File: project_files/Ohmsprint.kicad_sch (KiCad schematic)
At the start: 123 parts, among them J2 MEM2067-02-180-00-A, J3 PJ-002AH-SMT-TR, J4 SJ-3523-SMT-TR, J5 541324062, J6 USB4110-GF-A, Q1 SS8050, Q2 SS8050, Q3 AO3400A, SW1 SW_Push_1_Red, SW2 SW_Push_1_Red, SW3 SW_Push_2_Blue, U1 ESP32-WROOM-32E-N4, U2 AP63203WU, U3 AP63200WU, U4 ATM90E26-YU, U5 ABS210-13, U6 CP2102N-A02-GQFN28R, U7 MCP1727-3302E/SN, U8 TPS2121RUXR, U9 NHD-2.4-240320AF-CSXP, Y1 ABLS-8.192MHZ-B2-T

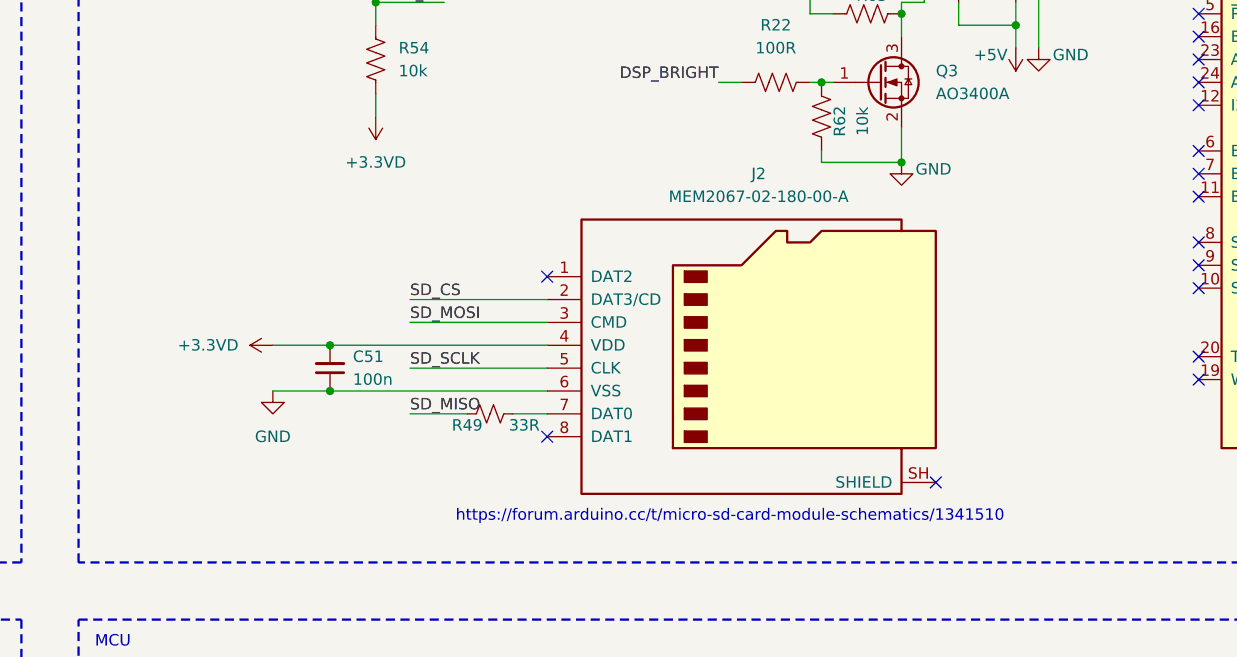
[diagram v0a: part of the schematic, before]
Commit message: Generisani Gerber i Drill
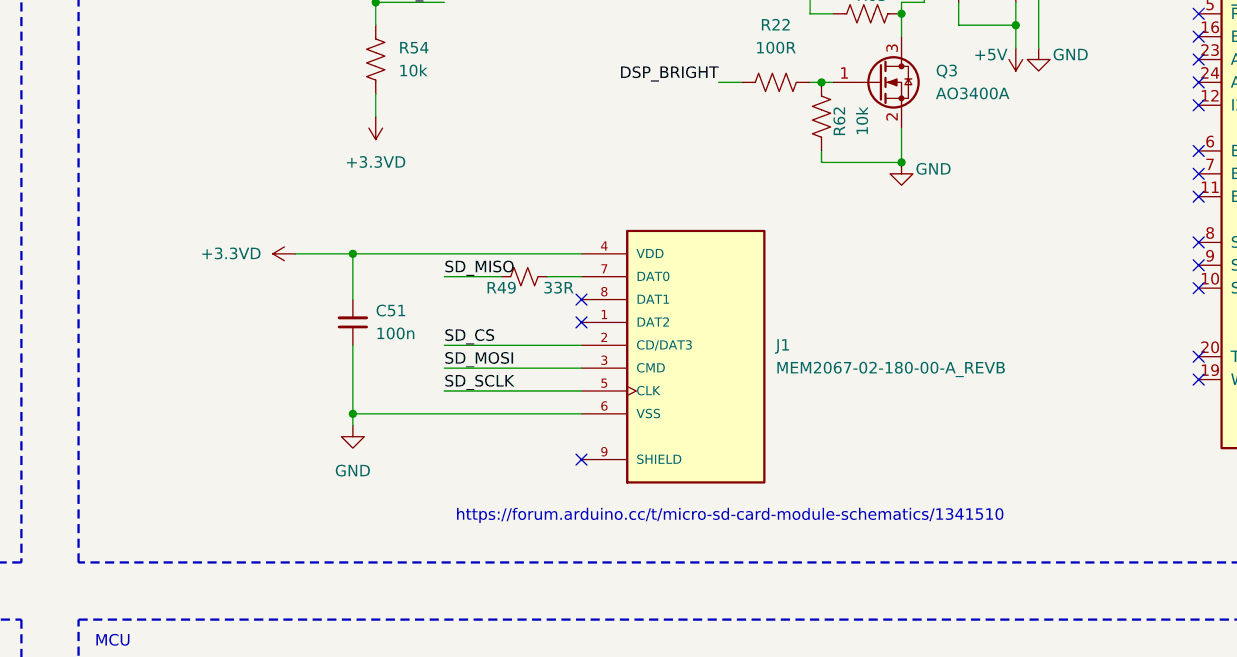
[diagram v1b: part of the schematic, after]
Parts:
- removed J2: MEM2067-02-180-00-A, usb:CONN_MEM2067-02-180-00-A_GCT, symbol Connector:Micro_SD_Card
- added J1: MEM2067-02-180-00-A_REVB, MEM2067-02-180-00-A_REVB_foot:GCT_MEM2067-02-180-00-A_REVB, symbol MEM2067-02-180-00-A_REVB:MEM2067-02-180-00-A_REVB
- J3: footprint PJ_002AH:PJ-002AH-SMT-TR_CUD -> CUI_PJ-002AH-SMT-TR-foot:CUI_PJ-002AH-SMT-TR
- J4: footprint SJ_3523_SMT:SJ-3523-SMT_CUD -> CUI_SJ-3523-SMT-TR-foot:CUI_SJ-3523-SMT-TR
- J5: footprint 541324062:CON_541324062_MOL -> Molex0541324062-foot:CON_541324062_MOL
- U1: footprint esp32_custom:ESP32-WROOM-32D -> RF_Module:ESP32-WROOM-32D
- U8: footprint TPS2121RUXR:RUX0012A -> TPS2121RUXR-foot:RUX0012A
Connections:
- net +3.3VD: now also J1.4 (VDD)
- net GND: now also J1.6 (VSS)
- net SD_CS: now also J1.2 (CD/DAT3)
- net SD_MOSI: now also J1.3 (CMD)
- net SD_SCLK: now also J1.5 (CLK)
- net at R49.2: now also J1.7 (DAT0)
- new net: J1.10 (SHIELD), J1.11 (SHIELD), J1.12 (SHIELD), J1.9 (SHIELD)
